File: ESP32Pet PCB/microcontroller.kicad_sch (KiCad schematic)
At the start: 2 parts, among them U2 ESP32-WROOM-32

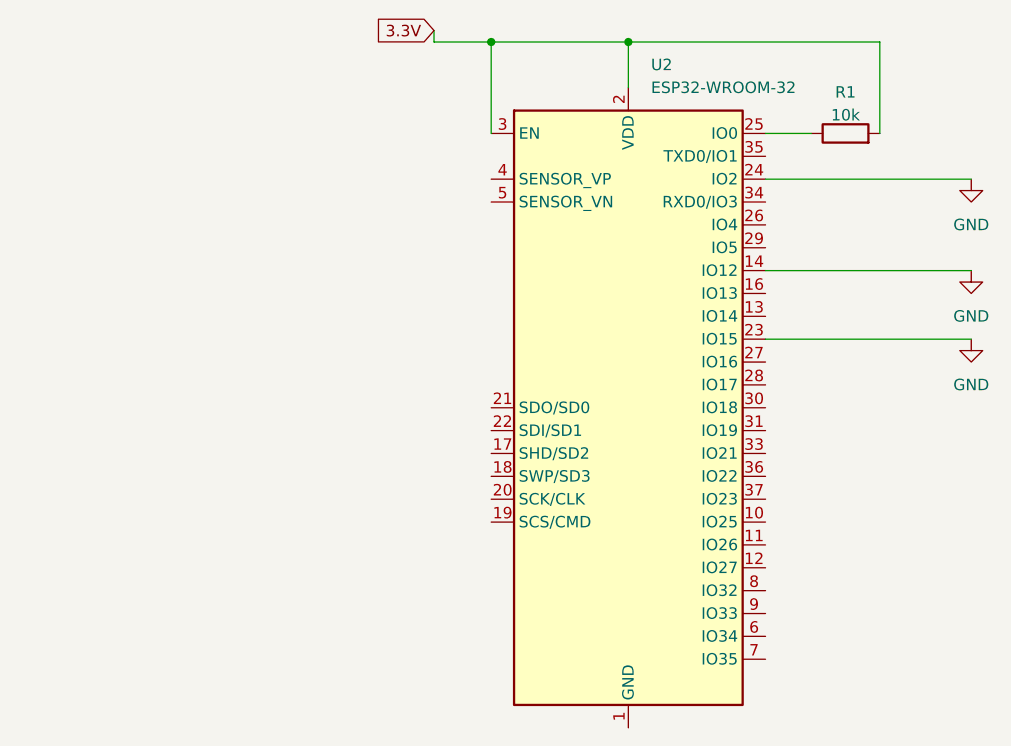
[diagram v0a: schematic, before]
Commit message: Schematic Updated
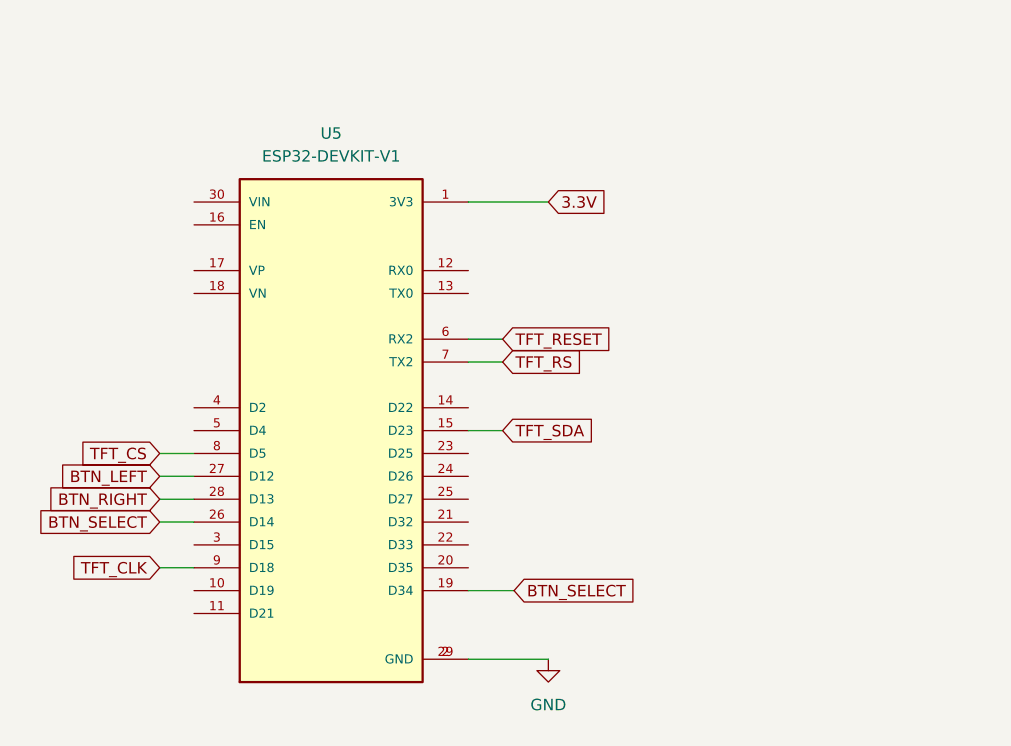
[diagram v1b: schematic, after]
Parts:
- removed R1: 10k, symbol Device:R
- removed U2: ESP32-WROOM-32, RF_Module:ESP32-WROOM-32, symbol RF_Module:ESP32-WROOM-32
- added U5: ESP32-DEVKIT-V1, ESP32-DEVKIT-V1:MODULE_ESP32_DEVKIT_V1, symbol ESP32-DEVKIT-V1:ESP32-DEVKIT-V1
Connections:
- net 3.3V: now also U5.1 (3V3)
- net GND: now also U5.2 (GND), U5.29 (GND)
- new net BTN_LEFT: U5.27 (D12)
- new net BTN_RIGHT: U5.28 (D13)
- new net BTN_SELECT: U5.19 (D34), U5.26 (D14)
- new net TFT_CLK: U5.9 (D18)
- new net TFT_CS: U5.8 (D5)
- new net TFT_RESET: U5.6 (RX2)
- new net TFT_RS: U5.7 (TX2)
- new net TFT_SDA: U5.15 (D23)

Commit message: Schematic complete, created custom footprints and symbols for TFT LCD
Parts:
- U5: footprint ESP32-DEVKIT-V1:MODULE_ESP32_DEVKIT_V1 -> ESP32 Devkit:MODULE_ESP32_DEVKIT_V1
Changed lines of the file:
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@@
+	(wire
+		(pts
+			(xy 128.27 69.85) (xy 124.46 69.85)
+		)
+		(stroke
+			(width 0)
+			(type default)
+		)
+	)
 	(wire
 		(pts
@@
 		(pts
 			(xy 124.46 72.39) (xy 128.27 72.39)
-		)
-		(stroke
-			(width 0)
-			(type default)
-		)
-	)
-	(wire
-		(pts
-			(xy 128.27 69.85) (xy 124.46 69.85)
 		)
 		(stroke
@@
 			)
 		)
-		(property "Footprint" "ESP32-DEVKIT-V1:MODULE_ESP32_DEVKIT_V1"
+		(property "Footprint" "ESP32 Devkit:MODULE_ESP32_DEVKIT_V1"
 			(at 109.22 80.01 0)
 			(effects
